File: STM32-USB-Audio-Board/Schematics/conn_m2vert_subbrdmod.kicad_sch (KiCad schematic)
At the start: 3 parts, among them CN501 Conn_02x38_Odd_Even

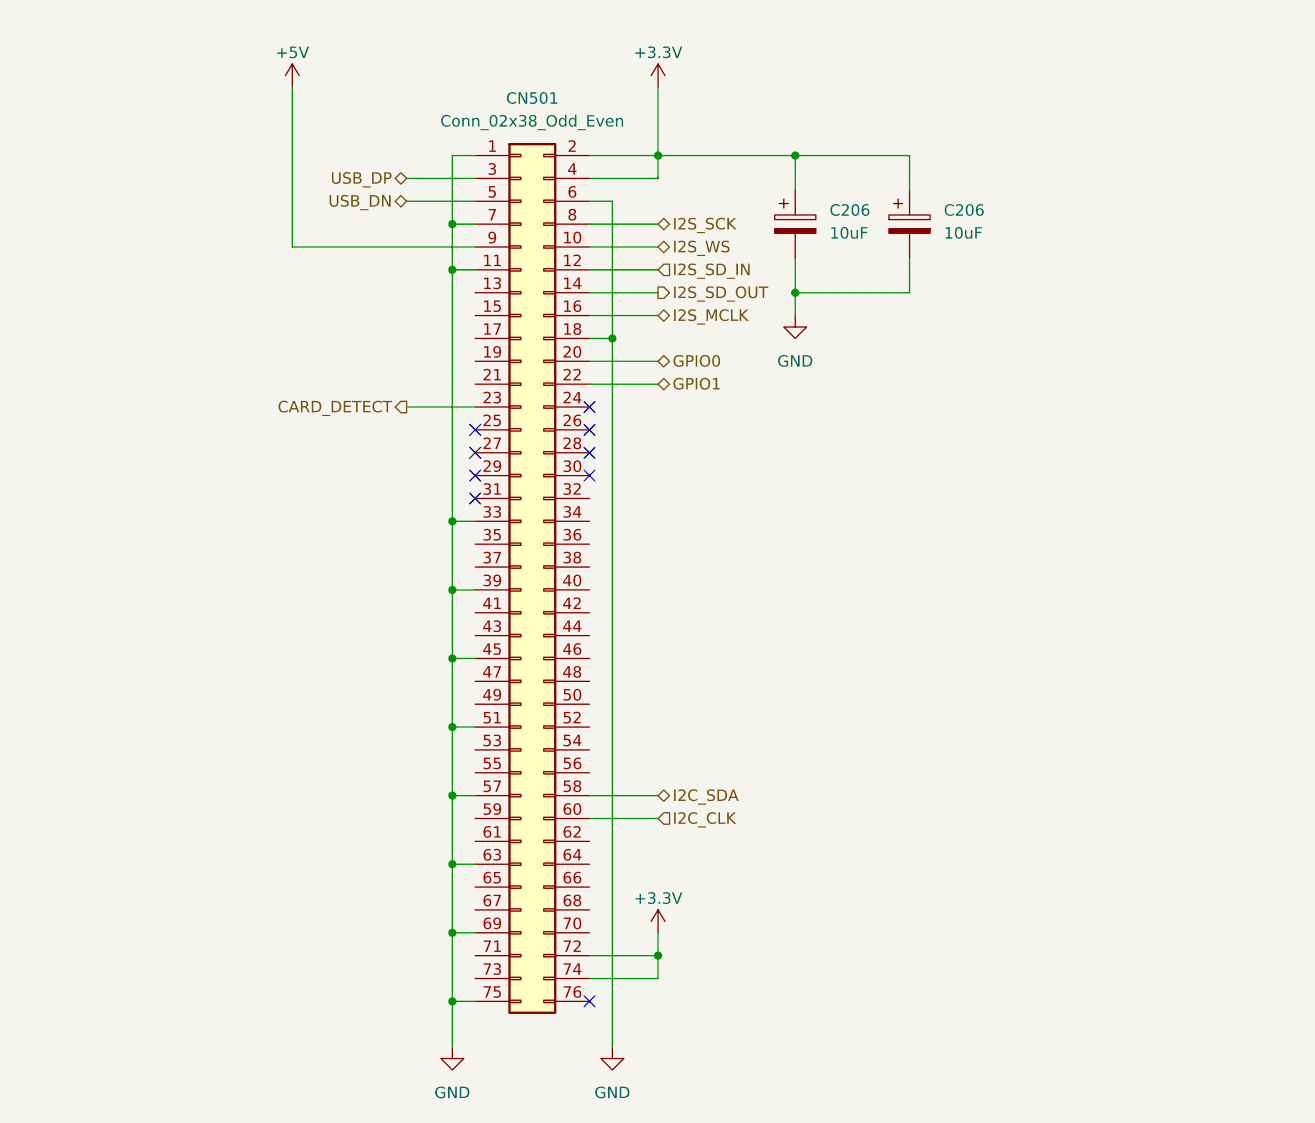
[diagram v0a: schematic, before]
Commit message: Cleanup
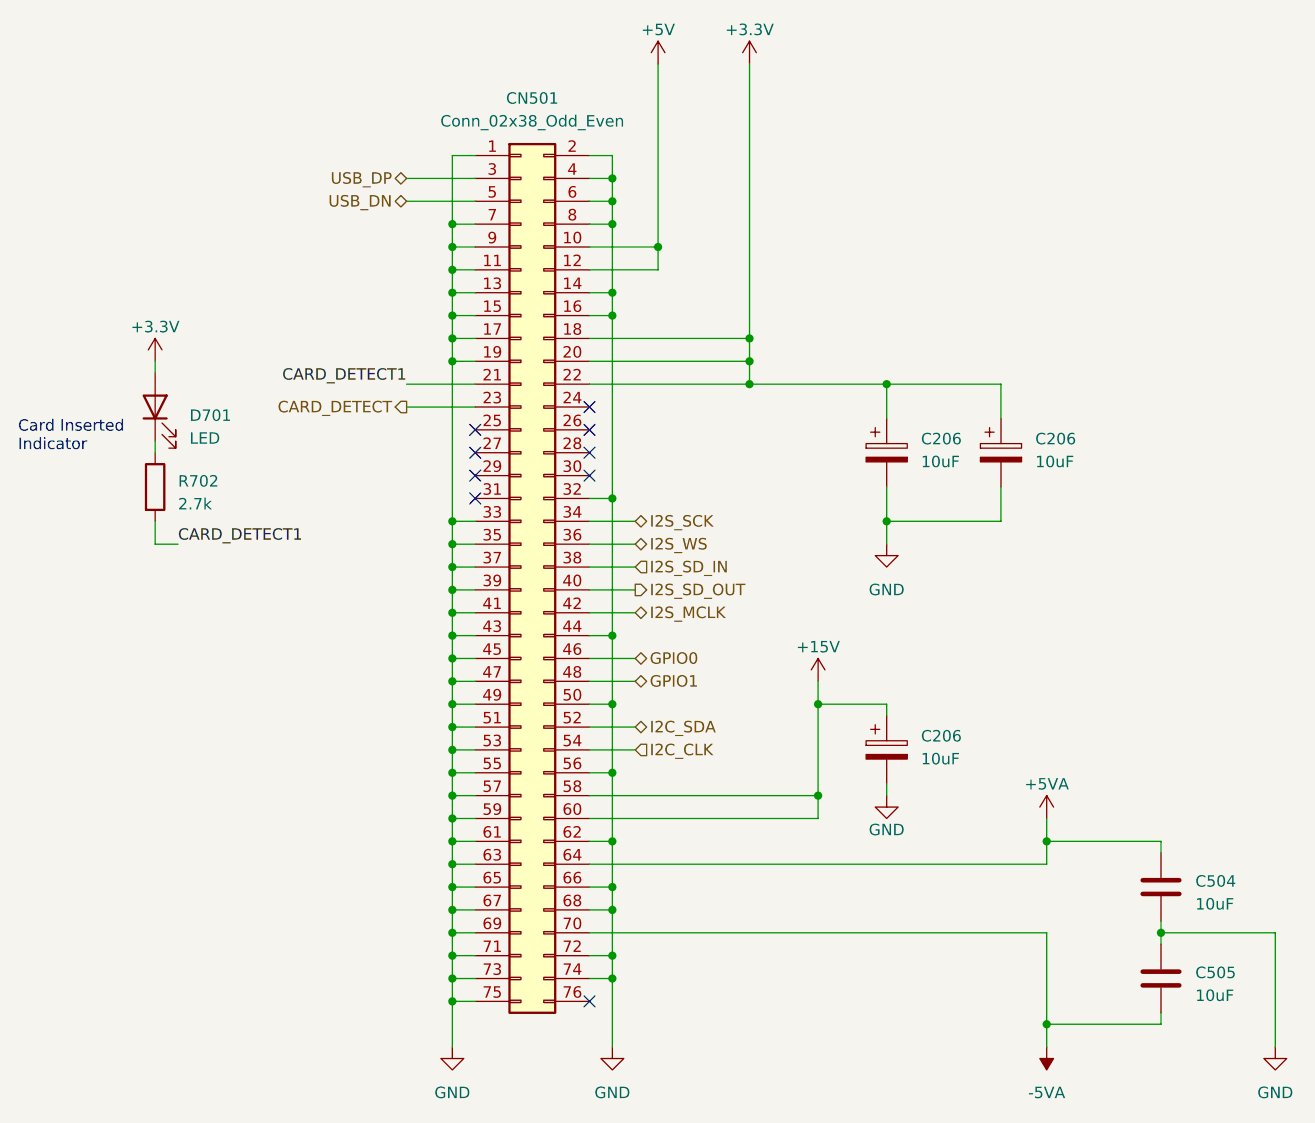
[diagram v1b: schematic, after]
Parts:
- added C206: 10uF, Capacitor_Tantalum_SMD:CP_EIA-3528-21_Kemet-B, symbol Device:C_Polarized
- added C504, C505: 10uF, Capacitor_SMD:C_0603_1608Metric, symbol Device:C
- added D701: LED, LED_SMD:LED_0603_1608Metric, symbol Device:LED
- added R702: 2.7k, Resistor_SMD:R_0402_1005Metric, symbol Device:R
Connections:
- net +3.3V: now also CN501.18 (Pin_18), CN501.20 (Pin_20), CN501.22 (Pin_22), D701.2 (A); no longer CN501.2 (Pin_2), CN501.4 (Pin_4), CN501.72 (Pin_72), CN501.74 (Pin_74)
- net +5V: now also CN501.10 (Pin_10), CN501.12 (Pin_12); no longer CN501.9 (Pin_9)
- net GND: now also CN501.13 (Pin_13), CN501.14 (Pin_14), CN501.15 (Pin_15), CN501.16 (Pin_16), CN501.17 (Pin_17), CN501.19 (Pin_19), CN501.2 (Pin_2), CN501.32 (Pin_32), CN501.35 (Pin_35), CN501.37 (Pin_37), CN501.4 (Pin_4), CN501.41 (Pin_41), CN501.43 (Pin_43), CN501.44 (Pin_44), CN501.47 (Pin_47), CN501.49 (Pin_49), CN501.50 (Pin_50), CN501.53 (Pin_53), CN501.55 (Pin_55), CN501.56 (Pin_56), CN501.59 (Pin_59), CN501.61 (Pin_61), CN501.62 (Pin_62), CN501.65 (Pin_65), CN501.66 (Pin_66), CN501.67 (Pin_67), CN501.68 (Pin_68), CN501.71 (Pin_71), CN501.72 (Pin_72), CN501.73 (Pin_73), CN501.74 (Pin_74), CN501.8 (Pin_8), CN501.9 (Pin_9), C206.2, C504.2, C505.1; no longer CN501.18 (Pin_18)
- net GPIO0: now also CN501.46 (Pin_46); no longer CN501.20 (Pin_20)
- net GPIO1: now also CN501.48 (Pin_48); no longer CN501.22 (Pin_22)
- net I2C_CLK: now also CN501.54 (Pin_54); no longer CN501.60 (Pin_60)
- net I2C_SDA: now also CN501.52 (Pin_52); no longer CN501.58 (Pin_58)
- net I2S_MCLK: now also CN501.42 (Pin_42); no longer CN501.16 (Pin_16)
- net I2S_SCK: now also CN501.34 (Pin_34); no longer CN501.8 (Pin_8)
- net I2S_SD_IN: now also CN501.38 (Pin_38); no longer CN501.12 (Pin_12)
- net I2S_SD_OUT: now also CN501.40 (Pin_40); no longer CN501.14 (Pin_14)
- net I2S_WS: now also CN501.36 (Pin_36); no longer CN501.10 (Pin_10)
- net CARD_DETECT1: now reaches CN501.21 (Pin_21)
- net CARD_DETECT1: now also R702.2
- net +5VA: now reaches CN501.64 (Pin_64)
- net +5VA: now also C504.1
- net -5VA: now reaches CN501.70 (Pin_70)
- net -5VA: now also C505.2
- new net: D701.1 (K), R702.1
- new net +15V: C206.1, CN501.58 (Pin_58), CN501.60 (Pin_60)
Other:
- note added: "Card Inserted Indicator"
- moved on the sheet: C206
